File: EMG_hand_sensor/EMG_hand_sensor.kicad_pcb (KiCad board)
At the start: 4 copper layers, 71.4 x 41.5 mm, 53 parts, among them J1 USB_C_Receptacle_USB2.0_16P, J2 Conn_01x04_Pin, J4 AudioJack3, J5 AudioJack3, J6 AudioJack3, SW1 SW_SPDT, U1 USBLC6-2SC6, U2 STM32F103C8Tx, U3 INA128, U5 INA128, U7 LT1762, U9 INA128, Y1 16MHz

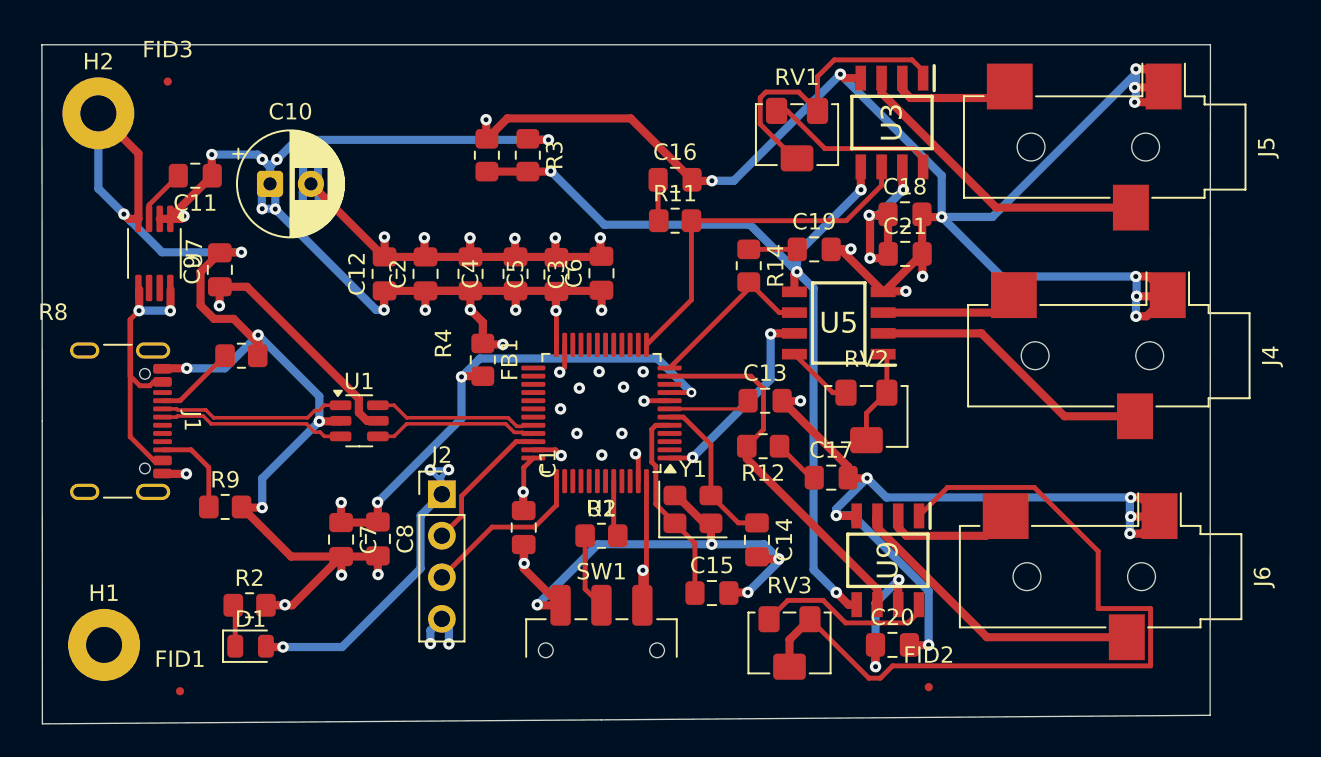
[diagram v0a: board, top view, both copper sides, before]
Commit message: done DRC final checks
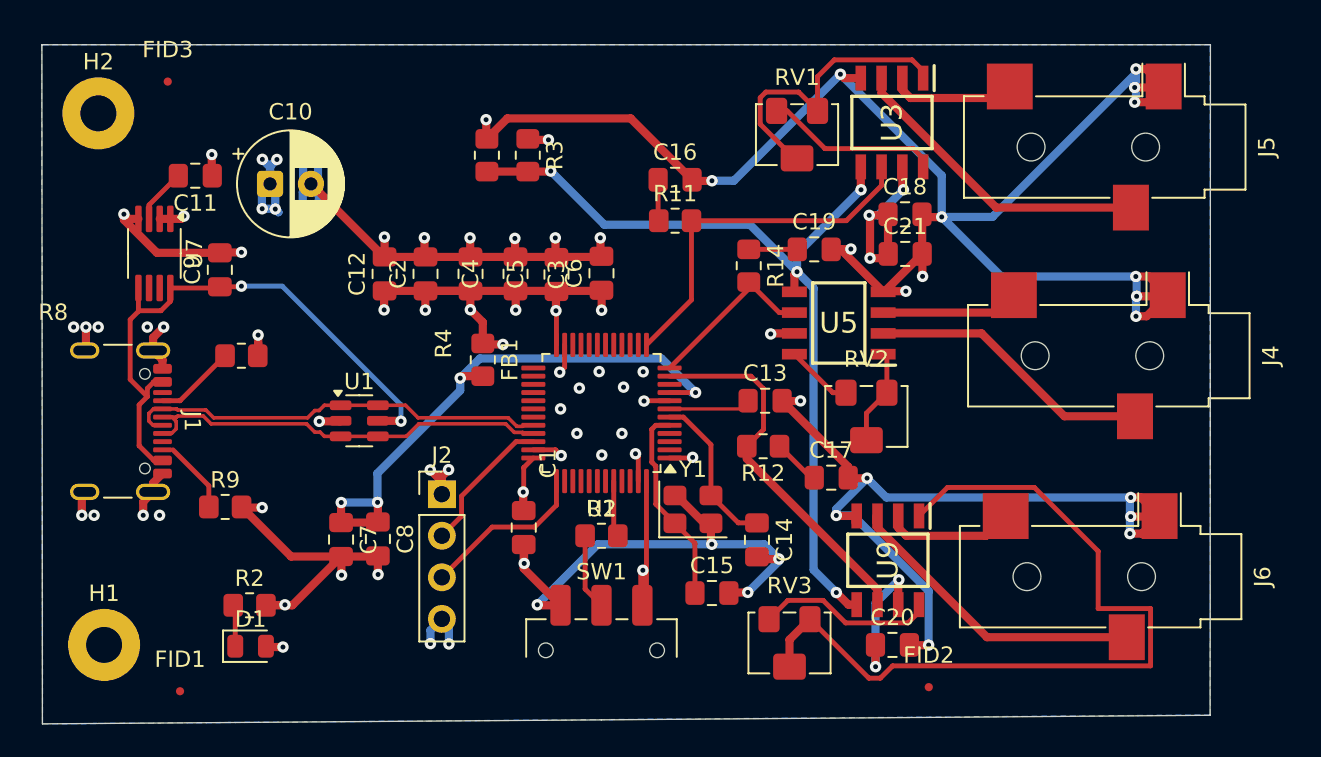
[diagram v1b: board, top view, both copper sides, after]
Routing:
- net +3.3V: track 142.3 -> 83.3 mm
- net GND: track 308.2 -> 271.5 mm, vias 59 -> 66
- net /USB_D-: track 21.5 -> 26.1 mm
- net /USB_D+: track 21.5 -> 26.1 mm
- net +3.3VA: track 32.5 -> 35.5 mm
- net /CC2: track 5.69 -> 4.40 mm
- net VBUS: track 36.5 -> 37.5 mm, vias 3 -> 2
- added copper zone on B.Cu, net +3.3V
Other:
- outline, holes or cut-outs redrawn
